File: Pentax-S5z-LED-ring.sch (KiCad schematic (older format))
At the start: 39 parts, among them IC1 ATTINY13-S, Q1 MOSFET_N, SW1 SW_PUSH, SW2 SW_PUSH

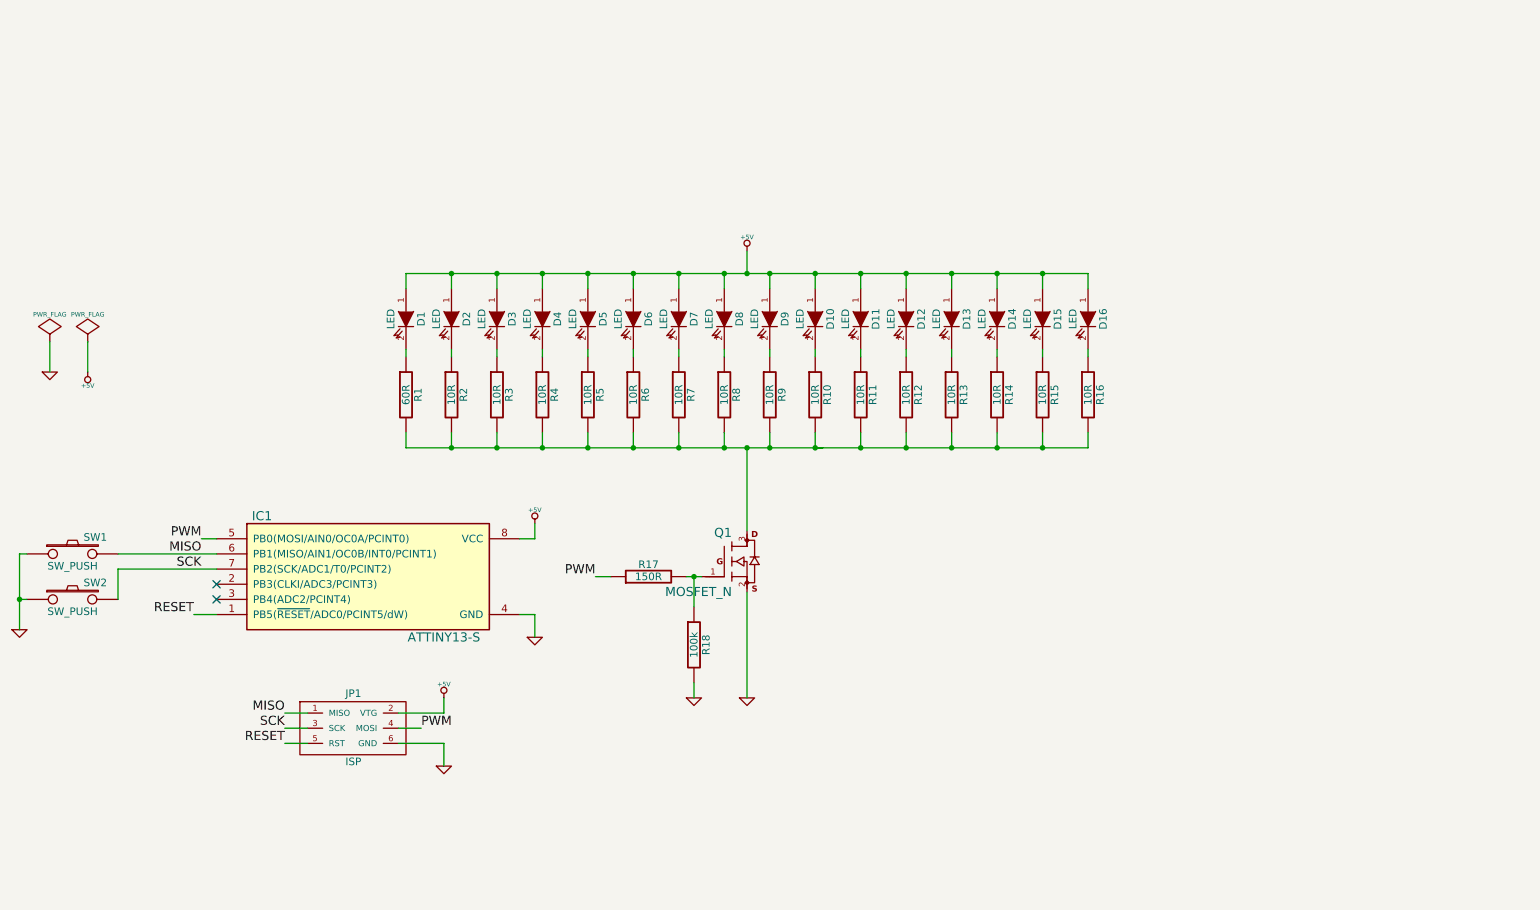
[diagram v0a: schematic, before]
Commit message: ...
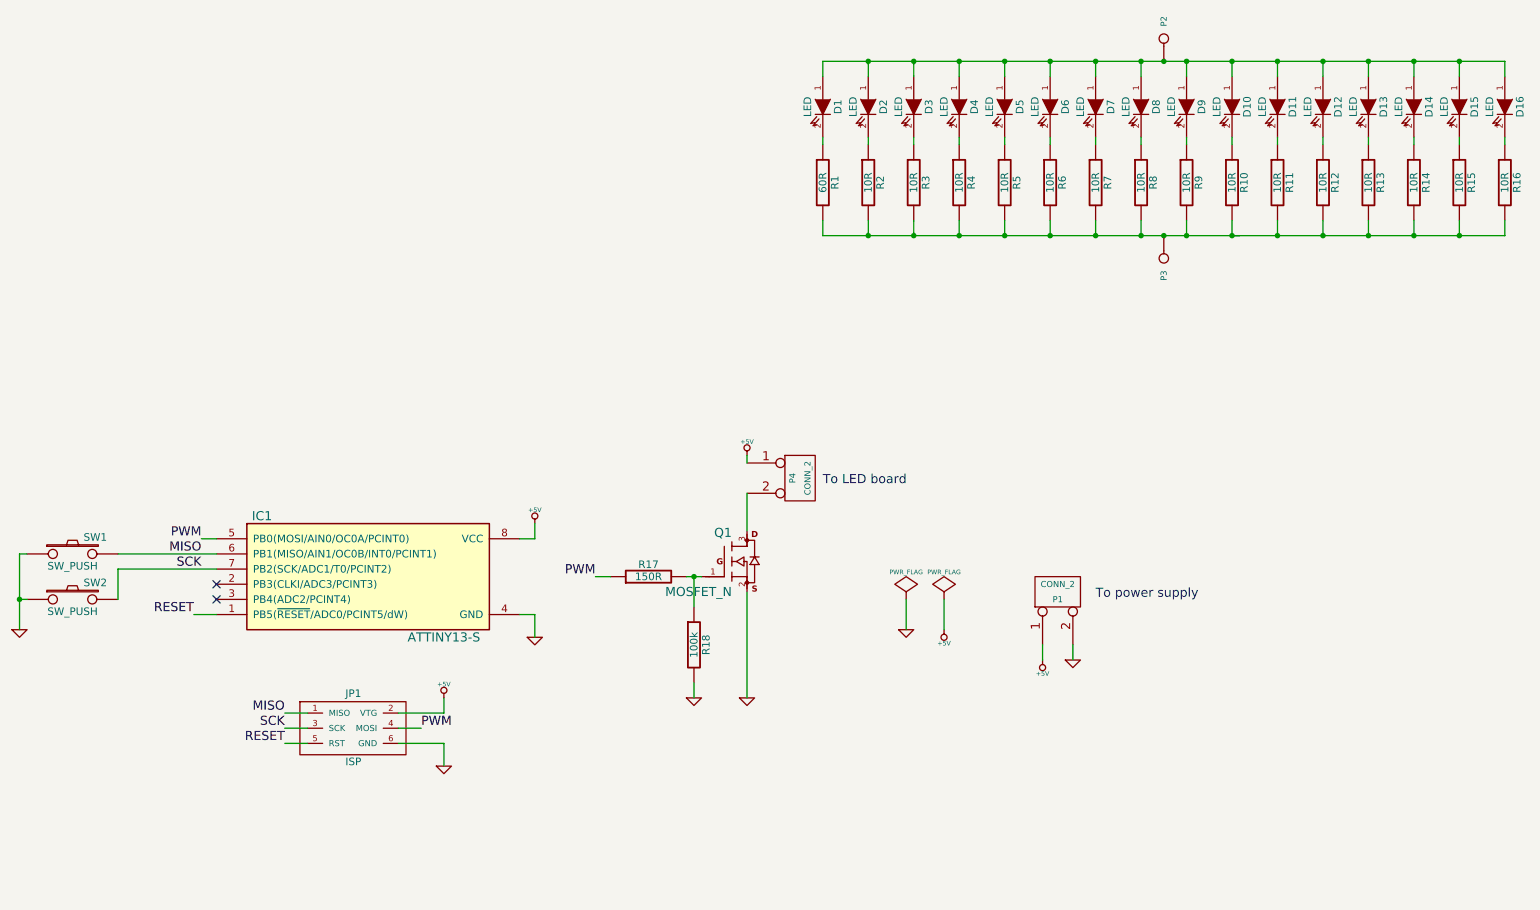
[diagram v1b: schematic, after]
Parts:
- added P1, P4: CONN_2, symbol CONN_2
- added P2: +, symbol CONN_1
- added P3: -, symbol CONN_1
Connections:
- net +5V: now also P1.1 (P1), P4.1 (P1); no longer D1.1 (A), D10.1 (A), D11.1 (A), D12.1 (A), D13.1 (A), D14.1 (A), D15.1 (A), D16.1 (A), D2.1 (A), D3.1 (A), D4.1 (A), D5.1 (A), D6.1 (A), D7.1 (A), D8.1 (A), D9.1 (A)
- net GND: now also P1.2 (PM)
- net at R1.2, R10.2, R11.2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: now also P3.1; no longer Q1.3 (D)
- new net: D1.1 (A), D10.1 (A), D11.1 (A), D12.1 (A), D13.1 (A), D14.1 (A), D15.1 (A), D16.1 (A), D2.1 (A), D3.1 (A), D4.1 (A), D5.1 (A), D6.1 (A), D7.1 (A), D8.1 (A), D9.1 (A), P2.1
- new net: P4.2 (PM), Q1.3 (D)
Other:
- note added: "To LED board"
- note added: "To power supply"
- moved on the sheet: D1, D10, D11, D12, D13, D14, D15, D16, D2, D3, D4, D5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

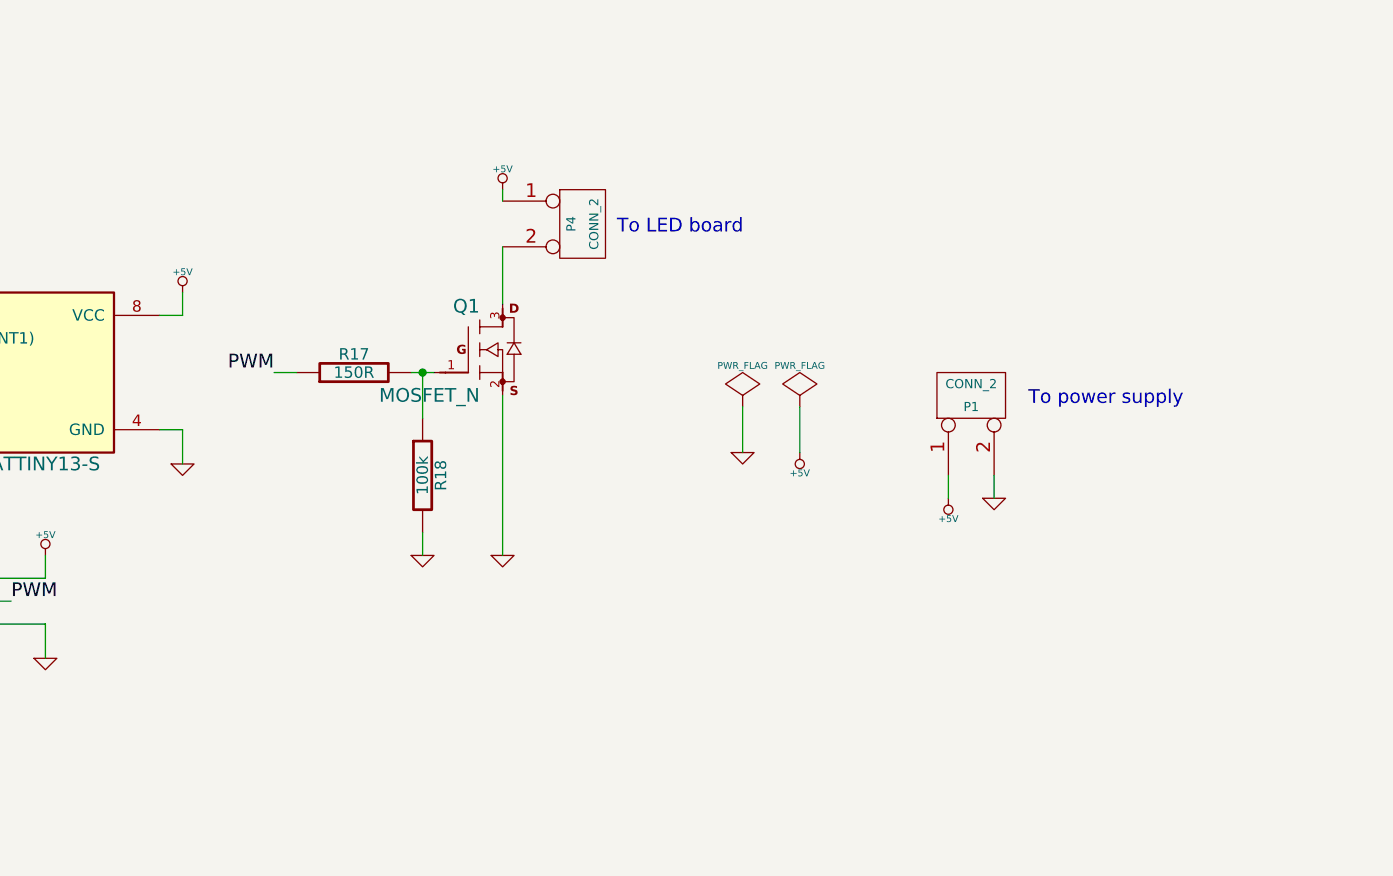
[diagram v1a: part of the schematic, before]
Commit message: Getting there...
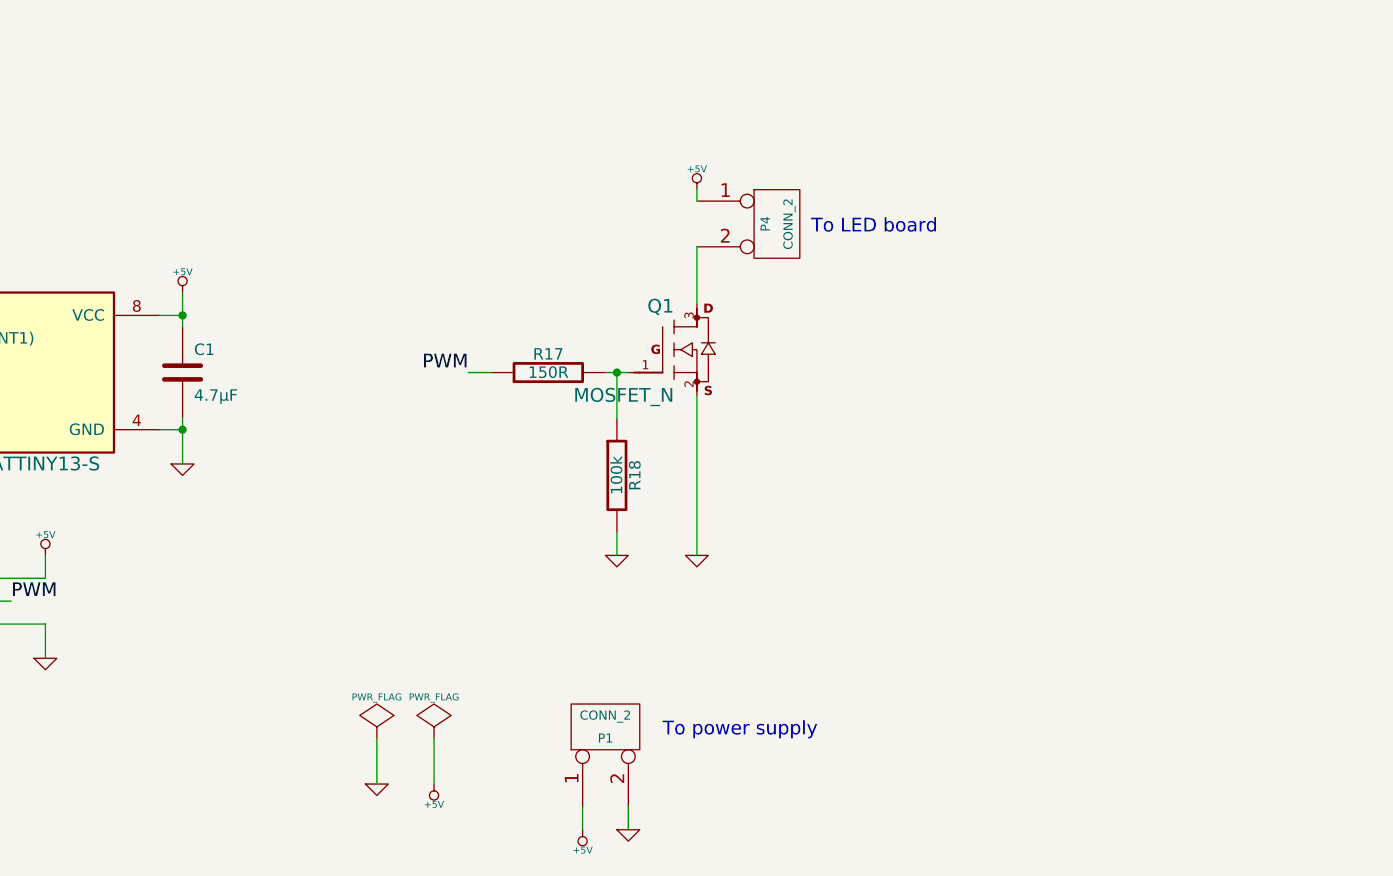
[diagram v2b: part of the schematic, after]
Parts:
- added C1: 4.7µF, symbol C
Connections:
- net +5V: now also C1.1
- net GND: now also C1.2
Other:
- moved on the sheet: P1, P4, Q1, R17, R18
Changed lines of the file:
@@
-EESchema Schematic File Version 2  date Tue 09 Apr 2013 09:44:23 PM CEST
+EESchema Schematic File Version 2  date Wed 10 Apr 2013 12:16:09 AM CEST
 LIBS:my_parts
 LIBS:power
@@
 L R R17
 U 1 1 51640F23
-P 5150 4450
-F 0 "R17" V 5230 4450 50  0000 C CNN
-F 1 "150R" V 5150 4450 50  0000 C CNN
-F 2 "" H 5150 4450 60  0000 C CNN
-F 3 "" H 5150 4450 60  0000 C CNN
-	1    5150 4450
+P 6000 4450
+F 0 "R17" V 6080 4450 50  0000 C CNN
+F 1 "150R" V 6000 4450 50  0000 C CNN
+F 2 "" H 6000 4450 60  0000 C CNN
+F 3 "" H 6000 4450 60  0000 C CNN
+	1    6000 4450
 	0    -1   -1   0
 $EndComp
@@
 L R R18
 U 1 1 51640F32
-P 5450 4900
-F 0 "R18" V 5530 4900 50  0000 C CNN
-F 1 "100k" V 5450 4900 50  0000 C CNN
-F 2 "" H 5450 4900 60  0000 C CNN
-F 3 "" H 5450 4900 60  0000 C CNN
-	1    5450 4900
+P 6300 4900
+F 0 "R18" V 6380 4900 50  0000 C CNN
+F 1 "100k" V 6300 4900 50  0000 C CNN
+F 2 "" H 6300 4900 60  0000 C CNN
+F 3 "" H 6300 4900 60  0000 C CNN
+	1    6300 4900
 	1    0    0    -1
 $EndComp
@@
 L MOSFET_N Q1
 U 1 1 51640F6E
-P 5500 4450
-F 0 "Q1" H 5700 4740 60  0000 R CNN
-F 1 "MOSFET_N" H 5700 4350 60  0000 R CNN
-F 2 "~" H 5500 4450 60  0000 C CNN
-F 3 "~" H 5500 4450 60  0000 C CNN
-	1    5500 4450
-	1    0    0    -1
-$EndComp
-Wire Wire Line
-	5400 4450 5500 4450
-Wire Wire Line
-	5450 4450 5450 4650
-Connection ~ 5450 4450
+P 6350 4450
+F 0 "Q1" H 6550 4740 60  0000 R CNN
+F 1 "MOSFET_N" H 6550 4350 60  0000 R CNN
+F 2 "~" H 6350 4450 60  0000 C CNN
+F 3 "~" H 6350 4450 60  0000 C CNN
+	1    6350 4450
+	1    0    0    -1
+$EndComp
+Wire Wire Line
+	6250 4450 6350 4450
+Wire Wire Line
+	6300 4450 6300 4650
+Connection ~ 6300 4450
 $Comp
 L GND #PWR01
 U 1 1 51641037
-P 5450 5250
-F 0 "#PWR01" H 5450 5250 30  0001 C CNN
-F 1 "GND" H 5450 5180 30  0001 C CNN
-F 2 "" H 5450 5250 60  0000 C CNN
-F 3 "" H 5450 5250 60  0000 C CNN
-	1    5450 5250
-	1    0    0    -1
-$EndComp
-Wire Wire Line
-	5450 5150 5450 5250
-Wire Wire Line
-	5800 4550 5800 5250
+P 6300 5250
+F 0 "#PWR01" H 6300 5250 30  0001 C CNN
+F 1 "GND" H 6300 5180 30  0001 C CNN
+F 2 "" H 6300 5250 60  0000 C CNN
+F 3 "" H 6300 5250 60  0000 C CNN
+	1    6300 5250
+	1    0    0    -1
+$EndComp
+Wire Wire Line
+	6300 5150 6300 5250
+Wire Wire Line
+	6650 4550 6650 5250
 $Comp
 L GND #PWR02
 U 1 1 51641142
-P 5800 5250
-F 0 "#PWR02" H 5800 5250 30  0001 C CNN
-F 1 "GND" H 5800 5180 30  0001 C CNN
-F 2 "" H 5800 5250 60  0000 C CNN
-F 3 "" H 5800 5250 60  0000 C CNN
-	1    5800 5250
+P 6650 5250
+F 0 "#PWR02" H 6650 5250 30  0001 C CNN
+F 1 "GND" H 6650 5180 30  0001 C CNN
+F 2 "" H 6650 5250 60  0000 C CNN
+F 3 "" H 6650 5250 60  0000 C CNN
+	1    6650 5250
 	1    0    0    -1
 $EndComp
@@
 $EndComp
 Wire Wire Line
-	4300 4200 4400 4200
-Wire Wire Line
-	4400 4200 4400 4100
+	4400 4100 4400 4250
 $Comp
 L GND #PWR05
@@
 $EndComp
 Wire Wire Line
-	4300 4700 4400 4700
-Wire Wire Line
-	4400 4700 4400 4850
-Text Label 4800 4450 2    60   ~ 0
+	4400 4650 4400 4850
+Text Label 5650 4450 2    60   ~ 0
 PWM
 Wire Wire Line
-	4800 4450 4900 4450
+	5650 4450 5750 4450
 Text Label 2200 4200 2    60   ~ 0
 PWM
@@
 L GND #PWR09
 U 1 1 51644384
-P 6850 4800
-F 0 "#PWR09" H 6850 4800 30  0001 C CNN
-F 1 "GND" H 6850 4730 30  0001 C CNN
-F 2 "" H 6850 4800 60  0000 C CNN
-F 3 "" H 6850 4800 60  0000 C CNN
-	1    6850 4800
+P 5250 6250
+F 0 "#PWR09" H 5250 6250 30  0001 C CNN
+F 1 "GND" H 5250 6180 30  0001 C CNN
+F 2 "" H 5250 6250 60  0000 C CNN
+F 3 "" H 5250 6250 60  0000 C CNN
+	1    5250 6250
 	1    0    0    -1
 $EndComp
@@
 L +5V #PWR010
 U 1 1 51644393
-P 7100 4800
-F 0 "#PWR010" H 7100 4890 20  0001 C CNN
-F 1 "+5V" H 7100 4890 30  0000 C CNN
-F 2 "" H 7100 4800 60  0000 C CNN
-F 3 "" H 7100 4800 60  0000 C CNN
-	1    7100 4800
+P 5500 6250
+F 0 "#PWR010" H 5500 6340 20  0001 C CNN
+F 1 "+5V" H 5500 6340 30  0000 C CNN
+F 2 "" H 5500 6250 60  0000 C CNN
+F 3 "" H 5500 6250 60  0000 C CNN
+	1    5500 6250
 	-1   0    0    1
 $EndComp
@@
 L PWR_FLAG #FLG011
 U 1 1 516443A2
-P 6850 4600
-F 0 "#FLG011" H 6850 4695 30  0001 C CNN
-F 1 "PWR_FLAG" H 6850 4780 30  0000 C CNN
-F 2 "" H 6850 4600 60  0000 C CNN
-F 3 "" H 6850 4600 60  0000 C CNN
-	1    6850 4600
+P 5250 6050
+F 0 "#FLG011" H 5250 6145 30  0001 C CNN
+F 1 "PWR_FLAG" H 5250 6230 30  0000 C CNN
+F 2 "" H 5250 6050 60  0000 C CNN
+F 3 "" H 5250 6050 60  0000 C CNN
+	1    5250 6050
 	1    0    0    -1
 $EndComp
@@
 L PWR_FLAG #FLG012
 U 1 1 516443B1
-P 7100 4600
-F 0 "#FLG012" H 7100 4695 30  0001 C CNN
-F 1 "PWR_FLAG" H 7100 4780 30  0000 C CNN
-F 2 "" H 7100 4600 60  0000 C CNN
-F 3 "" H 7100 4600 60  0000 C CNN
-	1    7100 4600
-	1    0    0    -1
-$EndComp
-Wire Wire Line
-	7100 4600 7100 4800
-Wire Wire Line
-	6850 4600 6850 4800
+P 5500 6050
+F 0 "#FLG012" H 5500 6145 30  0001 C CNN
+F 1 "PWR_FLAG" H 5500 6230 30  0000 C CNN
+F 2 "" H 5500 6050 60  0000 C CNN
+F 3 "" H 5500 6050 60  0000 C CNN
+	1    5500 6050
+	1    0    0    -1
+$EndComp
+Wire Wire Line
+	5500 6050 5500 6250
+Wire Wire Line
+	5250 6050 5250 6250
 $Comp
 L CONN_2 P1
 U 1 1 51646D70
-P 7850 4550
-F 0 "P1" V 7800 4550 40  0000 C CNN
-F 1 "CONN_2" V 7900 4550 40  0000 C CNN
-F 2 "" H 7850 4550 60  0000 C CNN
-F 3 "" H 7850 4550 60  0000 C CNN
-	1    7850 4550
+P 6250 6000
+F 0 "P1" V 6200 6000 40  0000 C CNN
+F 1 "CONN_2" V 6300 6000 40  0000 C CNN
+F 2 "" H 6250 6000 60  0000 C CNN
+F 3 "" H 6250 6000 60  0000 C CNN
+	1    6250 6000
 	0    -1   -1   0
 $EndComp
@@
 L GND #PWR013
 U 1 1 51646D84
-P 7950 5000
-F 0 "#PWR013" H 7950 5000 30  0001 C CNN
-F 1 "GND" H 7950 4930 30  0001 C CNN
-F 2 "" H 7950 5000 60  0000 C CNN
-F 3 "" H 7950 5000 60  0000 C CNN
-	1    7950 5000
+P 6350 6450
+F 0 "#PWR013" H 6350 6450 30  0001 C CNN
+F 1 "GND" H 6350 6380 30  0001 C CNN
+F 2 "" H 6350 6450 60  0000 C CNN
+F 3 "" H 6350 6450 60  0000 C CNN
+	1    6350 6450
 	1    0    0    -1
 $EndComp
@@
 L +5V #PWR014
 U 1 1 51646D93
-P 7750 5000
-F 0 "#PWR014" H 7750 5090 20  0001 C CNN
-F 1 "+5V" H 7750 5090 30  0000 C CNN
-F 2 "" H 7750 5000 60  0000 C CNN
-F 3 "" H 7750 5000 60  0000 C CNN
-	1    7750 5000
+P 6150 6450
+F 0 "#PWR014" H 6150 6540 20  0001 C CNN
+F 1 "+5V" H 6150 6540 30  0000 C CNN
+F 2 "" H 6150 6450 60  0000 C CNN
+F 3 "" H 6150 6450 60  0000 C CNN
+	1    6150 6450
 	-1   0    0    1
 $EndComp
 Wire Wire Line
-	7750 4900 7750 5000
-Wire Wire Line
-	7950 4900 7950 5000
+	6150 6350 6150 6450
+Wire Wire Line
+	6350 6350 6350 6450
 $Comp
 L CONN_1 P2
@@
 L CONN_2 P4
 U 1 1 51647217
-P 6150 3800
-F 0 "P4" V 6100 3800 40  0000 C CNN
-F 1 "CONN_2" V 6200 3800 40  0000 C CNN
-F 2 "" H 6150 3800 60  0000 C CNN
-F 3 "" H 6150 3800 60  0000 C CNN
-	1    6150 3800
-	1    0    0    -1
-$EndComp
-Wire Wire Line
-	5800 3900 5800 4150
+P 7000 3800
+F 0 "P4" V 6950 3800 40  0000 C CNN
+F 1 "CONN_2" V 7050 3800 40  0000 C CNN
+F 2 "" H 7000 3800 60  0000 C CNN
+F 3 "" H 7000 3800 60  0000 C CNN
+	1    7000 3800
+	1    0    0    -1
+$EndComp
+Wire Wire Line
+	6650 3900 6650 4150
 $Comp
 L +5V #PWR?
 U 1 1 516472A6
-P 5800 3650
-F 0 "#PWR?" H 5800 3740 20  0001 C CNN
-F 1 "+5V" H 5800 3740 30  0000 C CNN
-F 2 "" H 5800 3650 60  0000 C CNN
-F 3 "" H 5800 3650 60  0000 C CNN
-	1    5800 3650
-	1    0    0    -1
-$EndComp
-Wire Wire Line
-	5800 3650 5800 3700
-Text Notes 8100 4600 0    60   ~ 0
+P 6650 3650
+F 0 "#PWR?" H 6650 3740 20  0001 C CNN
+F 1 "+5V" H 6650 3740 30  0000 C CNN
+F 2 "" H 6650 3650 60  0000 C CNN
+F 3 "" H 6650 3650 60  0000 C CNN
+	1    6650 3650
+	1    0    0    -1
+$EndComp
+Wire Wire Line
+	6650 3650 6650 3700
+Text Notes 6500 6050 0    60   ~ 0
 To power supply
-Text Notes 6300 3850 0    60   ~ 0
+Text Notes 7150 3850 0    60   ~ 0
 To LED board
+Connection ~ 4400 4200
+Connection ~ 4400 4700
+$Comp
+L C C1
+U 1 1 516492F3
+P 4400 4450
+F 0 "C1" H 4450 4550 50  0000 L CNN
+F 1 "4.7µF" H 4450 4350 50  0000 L CNN
+F 2 "" H 4400 4450 60  0000 C CNN
+F 3 "" H 4400 4450 60  0000 C CNN
+	1    4400 4450
+	1    0    0    -1
+$EndComp
+Wire Wire Line
+	4300 4200 4400 4200
+Wire Wire Line
+	4300 4700 4400 4700
 $EndSCHEMATC
